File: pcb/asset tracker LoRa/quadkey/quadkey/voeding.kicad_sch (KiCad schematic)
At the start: 15 parts, among them J1 USB_B_Mini, U1 MCP73831, U2 TPS63001

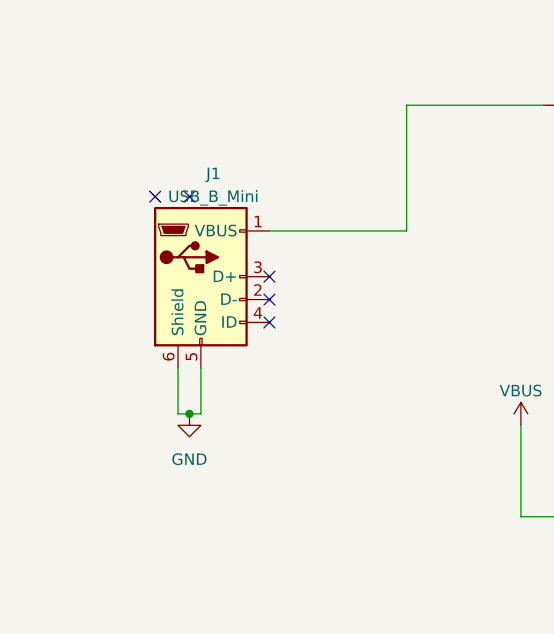
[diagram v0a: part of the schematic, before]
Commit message: code
code
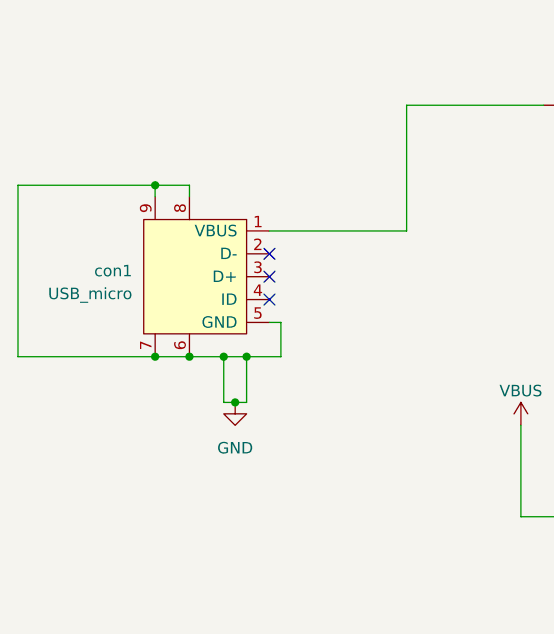
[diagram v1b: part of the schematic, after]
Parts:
- removed J1: USB_B_Mini, connectors_user:AMPHENOL_10118192-0001LF, symbol Connector:USB_B_Mini
- added con1: USB_micro, connectors_user:MILLMAX_897-43-005-00-100001, symbol conectors:USB_micro
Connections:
- net GND: now also con1.5 (GND), con1.6, con1.7, con1.8, con1.9
- net at L1.1: now also con1.1 (VBUS)
- no-connect marks 5 -> 3
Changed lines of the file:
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@@
     (comment 1 "bopla behuizing 34111511")
   )
-  (junction (at 43.18 63.5) (diameter 0.9144) (color 0 0 0 0))
+  (junction (at 39.37 38.1) (diameter 0.9144) (color 0 0 0 0))
+  (junction (at 39.37 57.15) (diameter 0.9144) (color 0 0 0 0))
+  (junction (at 43.18 57.15) (diameter 0.9144) (color 0 0 0 0))
+  (junction (at 46.99 57.15) (diameter 0.9144) (color 0 0 0 0))
+  (junction (at 48.26 62.23) (diameter 0.9144) (color 0 0 0 0))
+  (junction (at 49.53 57.15) (diameter 0.9144) (color 0 0 0 0))
   (junction (at 92.71 127) (diameter 0.9144) (color 0 0 0 0))
   (junction (at 104.14 29.21) (diameter 0.9144) (color 0 0 0 0))
@@
   (junction (at 190.5 147.32) (diameter 0.9144) (color 0 0 0 0))
   (junction (at 196.85 127) (diameter 0.9144) (color 0 0 0 0))
-  (no_connect (at 39.37 39.37))
-  (no_connect (at 43.18 39.37))
+  (no_connect (at 52.07 45.72))
   (no_connect (at 52.07 48.26))
   (no_connect (at 52.07 50.8))
-  (no_connect (at 52.07 53.34))
+  (wire (pts (xy 24.13 38.1) (xy 24.13 57.15))
+    (stroke (width 0) (type solid) (color 0 0 0 0))
+  )
+  (wire (pts (xy 24.13 57.15) (xy 39.37 57.15))
+    (stroke (width 0) (type solid) (color 0 0 0 0))
+  )
+  (wire (pts (xy 39.37 38.1) (xy 24.13 38.1))
+    (stroke (width 0) (type solid) (color 0 0 0 0))
+  )
+  (wire (pts (xy 39.37 38.1) (xy 43.18 38.1))
+    (stroke (width 0) (type solid) (color 0 0 0 0))
+  )
+  (wire (pts (xy 39.37 39.37) (xy 39.37 38.1))
+    (stroke (width 0) (type solid) (color 0 0 0 0))
+  )
   (wire (pts (xy 40.64 123.19) (xy 40.64 127))
     (stroke (width 0) (type solid) (color 0 0 0 0))
@@
     (stroke (width 0) (type solid) (color 0 0 0 0))
   )
-  (wire (pts (xy 41.91 63.5) (xy 41.91 58.42))
-    (stroke (width 0) (type solid) (color 0 0 0 0))
-  )
-  (wire (pts (xy 43.18 63.5) (xy 41.91 63.5))
-    (stroke (width 0) (type solid) (color 0 0 0 0))
-  )
-  (wire (pts (xy 44.45 58.42) (xy 44.45 63.5))
-    (stroke (width 0) (type solid) (color 0 0 0 0))
-  )
-  (wire (pts (xy 44.45 63.5) (xy 43.18 63.5))
+  (wire (pts (xy 43.18 39.37) (xy 43.18 38.1))
+    (stroke (width 0) (type solid) (color 0 0 0 0))
+  )
+  (wire (pts (xy 43.18 57.15) (xy 39.37 57.15))
+    (stroke (width 0) (type solid) (color 0 0 0 0))
+  )
+  (wire (pts (xy 46.99 57.15) (xy 43.18 57.15))
+    (stroke (width 0) (type solid) (color 0 0 0 0))
+  )
+  (wire (pts (xy 46.99 62.23) (xy 46.99 57.15))
+    (stroke (width 0) (type solid) (color 0 0 0 0))
+  )
+  (wire (pts (xy 48.26 62.23) (xy 46.99 62.23))
+    (stroke (width 0) (type solid) (color 0 0 0 0))
+  )
+  (wire (pts (xy 49.53 57.15) (xy 46.99 57.15))
+    (stroke (width 0) (type solid) (color 0 0 0 0))
+  )
+  (wire (pts (xy 49.53 57.15) (xy 49.53 62.23))
+    (stroke (width 0) (type solid) (color 0 0 0 0))
+  )
+  (wire (pts (xy 49.53 62.23) (xy 48.26 62.23))
+    (stroke (width 0) (type solid) (color 0 0 0 0))
+  )
+  (wire (pts (xy 52.07 53.34) (xy 53.34 53.34))
+    (stroke (width 0) (type solid) (color 0 0 0 0))
+  )
+  (wire (pts (xy 53.34 53.34) (xy 53.34 57.15))
+    (stroke (width 0) (type solid) (color 0 0 0 0))
+  )
+  (wire (pts (xy 53.34 57.15) (xy 49.53 57.15))
     (stroke (width 0) (type solid) (color 0 0 0 0))
   )
@@
     (pin "1")
   )
-  (symbol (lib_id "power:GND") (at 43.18 63.5 0) (unit 1)
-    (in_bom yes) (on_board yes) (fields_autoplaced)
-    (property "Reference" "#PWR0104" (id 0) (at 43.18 69.85 0)
-      (effects (font (size 1.27 1.27)) hide)
-    )
-    (property "Value" "GND" (id 1) (at 43.18 68.58 0))
-    (property "Footprint" "" (id 2) (at 43.18 63.5 0)
-      (effects (font (size 1.27 1.27)) hide)
-    )
-    (property "Datasheet" "" (id 3) (at 43.18 63.5 0)
+  (symbol (lib_id "power:GND") (at 48.26 62.23 0) (unit 1)
+    (in_bom yes) (on_board yes) (fields_autoplaced)
+    (property "Reference" "#PWR0104" (id 0) (at 48.26 68.58 0)
+      (effects (font (size 1.27 1.27)) hide)
+    )
+    (property "Value" "GND" (id 1) (at 48.26 67.31 0))
+    (property "Footprint" "" (id 2) (at 48.26 62.23 0)
+      (effects (font (size 1.27 1.27)) hide)
+    )
+    (property "Datasheet" "" (id 3) (at 48.26 62.23 0)
       (effects (font (size 1.27 1.27)) hide)
     )
@@
     (pin "5")
   )
-  (symbol (lib_id "Connector:USB_B_Mini") (at 44.45 48.26 0) (unit 1)
-    (in_bom yes) (on_board yes) (fields_autoplaced)
-    (property "Reference" "J1" (id 0) (at 45.847 36.83 0))
-    (property "Value" "USB_B_Mini" (id 1) (at 45.847 39.37 0))
-    (property "Footprint" "connectors_user:AMPHENOL_10118192-0001LF" (id 2) (at 48.26 49.53 0)
-      (effects (font (size 1.27 1.27)) hide)
-    )
-    (property "Datasheet" "" (id 3) (at 48.26 49.53 0)
+  (symbol (lib_id "conectors:USB_micro") (at 49.53 43.18 0) (mirror y) (unit 1)
+    (in_bom yes) (on_board yes) (fields_autoplaced)
+    (property "Reference" "con1" (id 0) (at 36.83 47.6249 0)
+      (effects (font (size 1.27 1.27)) (justify left))
+    )
+    (property "Value" "USB_micro" (id 1) (at 36.83 50.1649 0)
+      (effects (font (size 1.27 1.27)) (justify left))
+    )
+    (property "Footprint" "connectors_user:MILLMAX_897-43-005-00-100001" (id 2) (at 49.53 43.18 0)
+      (effects (font (size 1.27 1.27)) hide)
+    )
+    (property "Datasheet" "" (id 3) (at 49.53 43.18 0)
       (effects (font (size 1.27 1.27)) hide)
     )
@@
     (pin "5")
     (pin "6")
+    (pin "7")
+    (pin "8")
+    (pin "9")
   )
   (symbol (lib_id "Regulator_Switching:TPS63001") (at 146.05 132.08 0) (unit 1)
